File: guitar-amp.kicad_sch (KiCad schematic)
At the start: 44 parts, among them U1 ECC81, U2 ECC81, U3 EL84

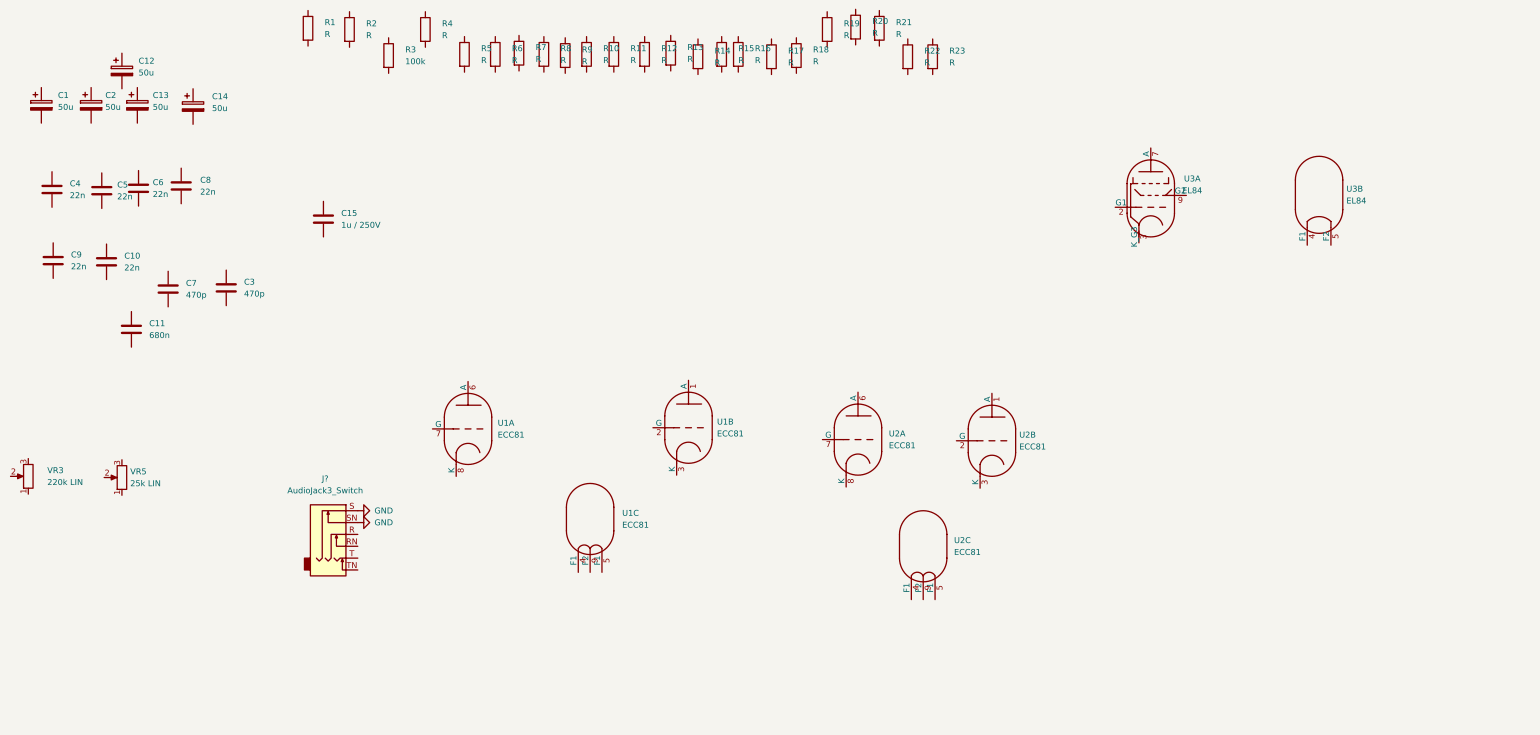
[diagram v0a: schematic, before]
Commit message: Model the schematic
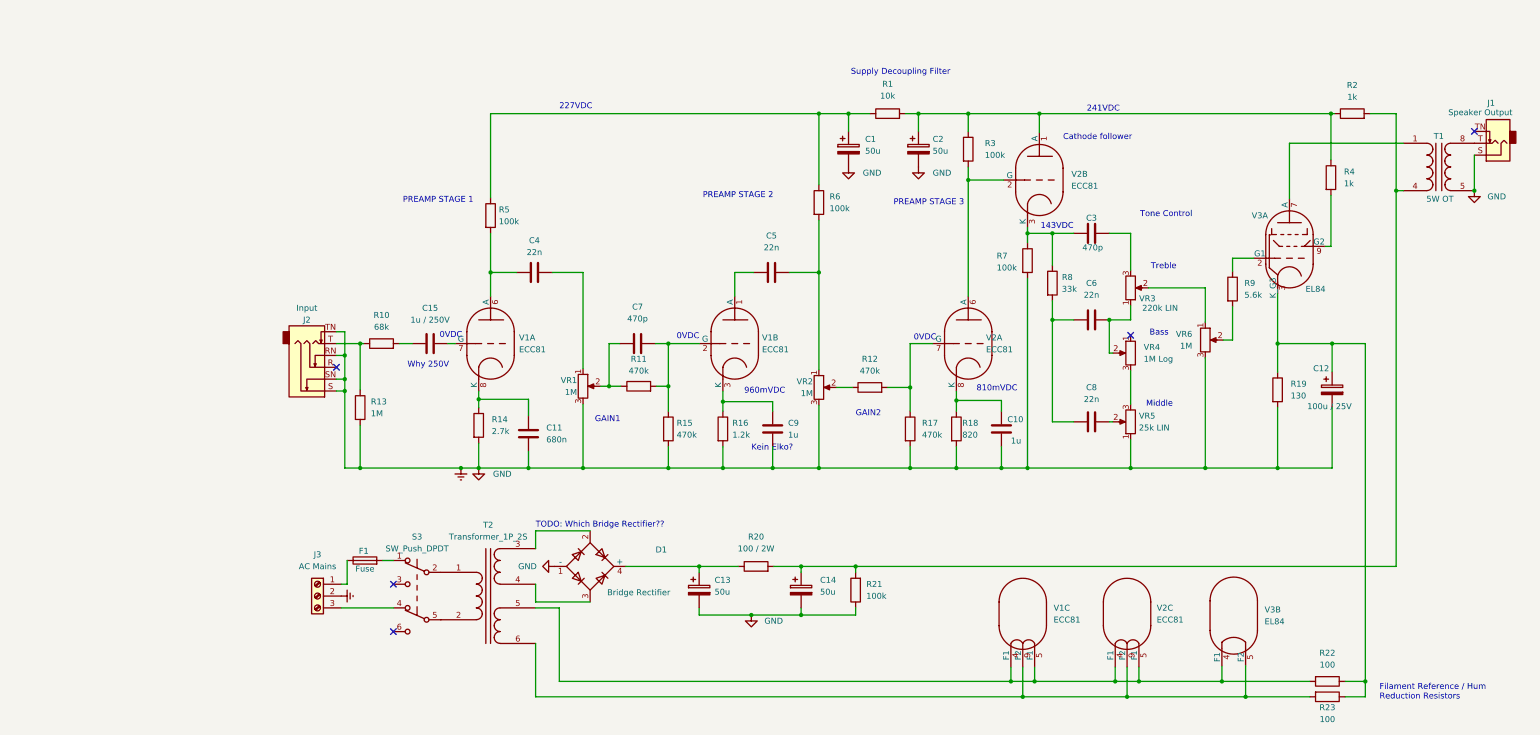
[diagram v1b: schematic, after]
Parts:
- added D1: Bridge Rectifier, Diode_THT:Diode_Bridge_32.0x5.6x17.0mm_P10.0mm_P7.5mm, symbol Diode_Bridge:B40C3x00-2200A
- added F1: Fuse, Fuse:Fuseholder_Cylinder-5x20mm_Schurter_0031_8201_Horizontal_Open, symbol Device:Fuse
- added J1: Speaker Output, TerminalBlock_Phoenix:TerminalBlock_Phoenix_MKDS-1,5-2-5.08_1x02_P5.08mm_Horizontal, symbol Connector:AudioJack2_SwitchT
- added J3: AC Mains, symbol Connector:Screw_Terminal_01x03
- added S3: SW_Push_DPDT, Button_Switch_THT:SW_CuK_JS202011CQN_DPDT_Straight, symbol Switch:SW_Push_DPDT
- added T1: 5W OT, symbol Device:Transformer_1P_1S_SO8
- added T2: Transformer_1P_2S, symbol Device:Transformer_1P_2S
- added VR1, VR2, VR6: 1M, Potentiometer_THT:Potentiometer_Piher_PT-15-V15_Vertical, symbol Device:R_Potentiometer
- added VR4: 1M Log, Potentiometer_THT:Potentiometer_Piher_PT-15-V15_Vertical, symbol Device:R_Potentiometer
- C10, C9: value 22n -> 1u
- C12: value 50u -> 100u / 25V
- J2: renamed from J?; value AudioJack3_Switch -> Input
- R1: value R -> 10k
- R10: value R -> 68k
- R11, R12, R15, R17: value R -> 470k
- R13: value R -> 1M
- R14: value R -> 2.7k
- R16: value R -> 1.2k
- R18: value R -> 820
- R19: value R -> 130
- R2, R4: value R -> 1k
- R20: value R -> 100 / 2W
- R21, R5, R6, R7: value R -> 100k
- R22, R23: value R -> 100
- R8: value R -> 33k
- R9: value R -> 5.6k
- renumbered U1 to V1, U2 to V2, U3 to V3
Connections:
- net GND is gone; now on net Earth: J2.S, J2.SN
- net at C9.1: now also R16.1, V1.3 (K)
- net Earth: now reaches C9.2
- net Earth: now also C1.2, C10.2, C11.2, C12.2, C13.2, C14.2, C2.2, J2.RN, J2.TN, R13.2, R14.2, R15.2, R16.2, R17.2, R18.2, R19.2, R21.1, R7.2, VR5.1, D1.1 (-), J1.S, J3.2 (Pin_2), T1.5 (SA), VR1.3, VR2.3, VR6.3
- net at V1.1 (A): now also C5.1
- net at V1.2 (G): now also C7.2, R11.2, R15.1
- net at R2.1: now also C2.1, R1.2, R3.1, R4.1, V2.1 (A)
- net at R2.2: now also C14.1, R20.2, R21.2, T1.4 (AB)
- net at R10.1: now also J2.T, R13.1
- net at R10.2: now also C15.1
- net at C4.1: now also R5.2, V1.6 (A)
- net at C4.2: now also VR1.1
- net at C11.1: now also R14.1, V1.8 (K)
- net at R17.1: now also R12.2, V2.7 (G)
- net at V1.7 (G): now also C15.2
- net at R9.1: now also V3.2 (G1)
- net at R9.2: now also VR6.2
- net at V3.4 (F1): now also R22.2, V1.4 (F1), V1.5 (F1), V2.4 (F1), V2.5 (F1), T2.5 (SC)
- net at V3.5 (F2): now also R23.2, V1.9 (F2), V2.9 (F2), T2.6 (SD)
- net at R8.1: now also C3.1, R7.1, V2.3 (K)
- net at R8.2: now also C6.1, C8.1
- net at VR5.2: now also C8.2
- net at VR5.3: now also VR4.3
- net at C10.1: now also R18.1, V2.8 (K)
- net at V2.2 (G): now also R3.2, V2.6 (A)
- net at R20.1: now also C13.1, D1.4 (+)
- net at C5.2: now also R6.2, VR2.1
- net at R22.1: now also C12.1, R19.1, R23.1, V3.3 (K_G3)
- net at R6.1: now also C1.1, R1.1, R5.1
- net at R12.1: now also VR2.2
- net at V3.7 (A): now also T1.1 (AA)
- net at V3.9 (G2): now also R4.2
- net at C3.2: now also VR3.3
- net at R11.1: now also C7.1, VR1.2
- net at C6.2: now also VR3.1, VR4.2
- net at VR3.2: now also VR6.1
- new net: D1.2, T2.3 (SA)
- new net: D1.3, T2.4 (SB)
- new net: J1.T, T1.8 (SB)
- new net: F1.1, J3.1 (Pin_1)
- new net: F1.2, S3.1 (A)
- new net: S3.2 (B), T2.1 (AA)
- new net: S3.5 (B), T2.2 (AB)
- new net: J3.3 (Pin_3), S3.4 (A)
- no-connect marks 0 -> 5
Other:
- note added: "0VDC"
- note added: "143VDC"
- note added: "227VDC"
- note added: "241VDC"
- note added: "810mVDC"
- note added: "960mVDC"
- note added: "Bass"
- note added: "Cathode follower"
- note added: "Filament Reference / Hum Reduction Resistors"
- note added: "GAIN1"
- note added: "GAIN2"
- note added: "Kein Elko?"
- note added: "Middle"
- note added: "PREAMP STAGE 1"
- note added: "PREAMP STAGE 2"
- note added: "PREAMP STAGE 3"
- note added: "Supply Decoupling Filter"
- note added: "TODO: Which Bridge Rectifier??"
- note added: "Tone Control"
- note added: "Treble"
- note added: "Why 250V"
- moved on the sheet: C1, C10, C11, C12, C13, C14, C15, C2, C3, C4, C5, C6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
